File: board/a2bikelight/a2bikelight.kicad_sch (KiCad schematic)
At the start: 1 part

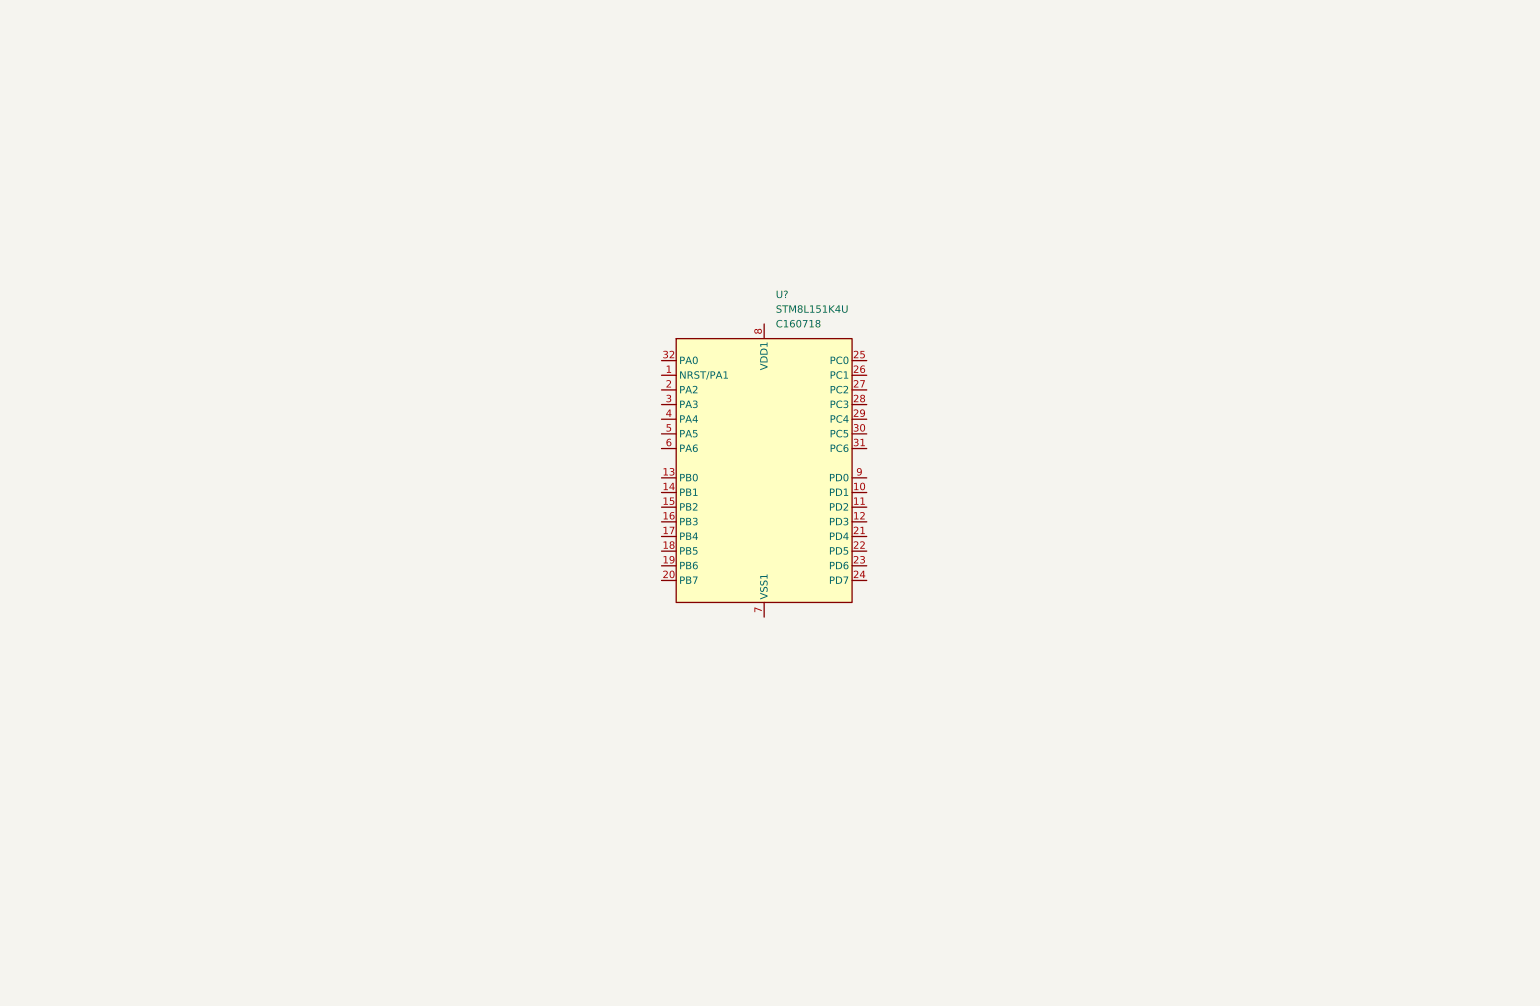
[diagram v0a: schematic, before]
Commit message: baseline
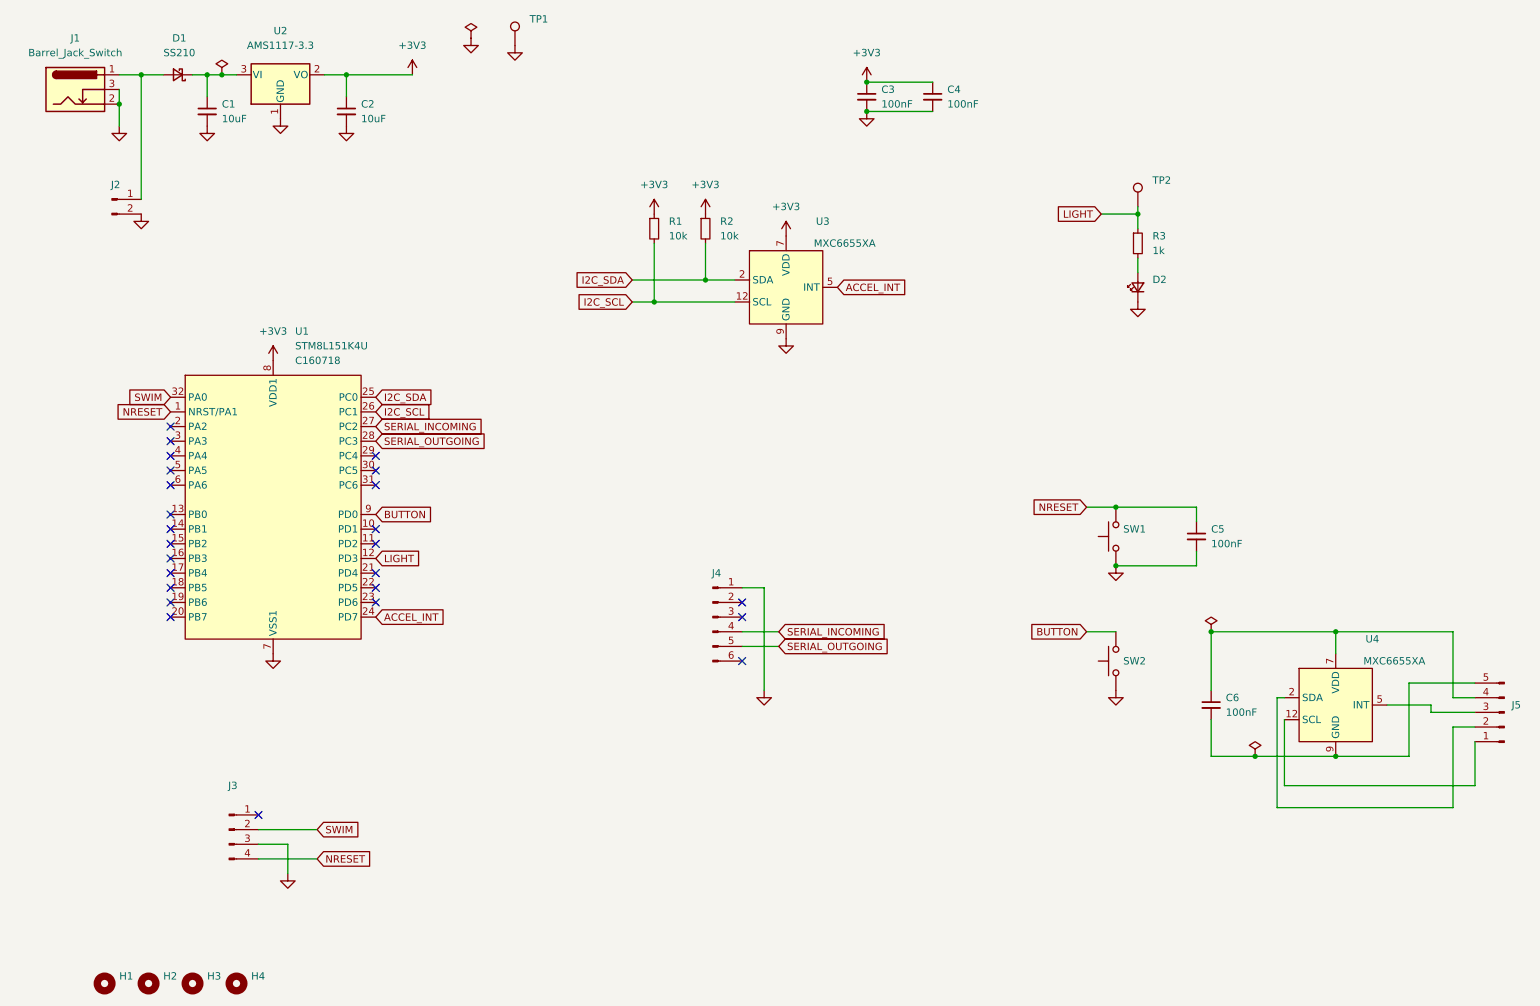
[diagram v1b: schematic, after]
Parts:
- added C1, C2: 10uF, Capacitor_SMD:C_0603_1608Metric, symbol Device:C_Small
- added C3, C4, C5, C6: 100nF, Capacitor_SMD:C_0603_1608Metric, symbol Device:C_Small
- added D1: SS210, Diode_SMD:D_SMA, symbol Device:D_Schottky_Small
- added D2: LED_Small, LED_SMD:LED_0805_2012Metric, symbol Device:LED_Small
- added H1, H2, H3, H4: MountingHole, MountingHole:MountingHole_3.5mm, symbol Mechanical:MountingHole
- added J1: Barrel_Jack_Switch, Connector_BarrelJack:BarrelJack_Horizontal, symbol Connector:Barrel_Jack_Switch
- added J2: Conn_01x02_Male, Connector_PinHeader_2.54mm:PinHeader_1x02_P2.54mm_Vertical, symbol Connector:Conn_01x02_Male
- added J3: Conn_01x04_Male, Connector_PinHeader_2.54mm:PinHeader_1x04_P2.54mm_Vertical, symbol Connector:Conn_01x04_Male
- added J4: Conn_01x06_Male, Connector_PinHeader_2.54mm:PinHeader_1x06_P2.54mm_Vertical, symbol Connector:Conn_01x06_Male
- added J5: Conn_01x05_Male, Connector_PinHeader_2.54mm:PinHeader_1x05_P2.54mm_Vertical, symbol Connector:Conn_01x05_Male
- added R1, R2: 10k, Resistor_SMD:R_0603_1608Metric, symbol Device:R_Small
- added R3: 1k, Resistor_SMD:R_0603_1608Metric, symbol Device:R_Small
- added SW1, SW2: SW_Push, Button_Switch_THT:SW_PUSH_6mm, symbol Switch:SW_Push
- added TP1, TP2: TestPoint, TestPoint:TestPoint_THTPad_2.0x2.0mm_Drill1.0mm, symbol Connector:TestPoint
- added U2: AMS1117-3.3, Package_TO_SOT_SMD:SOT-223-3_TabPin2, symbol Regulator_Linear:AMS1117-3.3
- added U3, U4: MXC6655XA, Package_LGA:LGA-12_2x2mm_P0.5mm, symbol a2bikelight:MXC6655XA
- gave numbers to parts that had none: 1
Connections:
- net NRESET: now reaches U1.1 (NRST/PA1)
- net NRESET: now also C5.1, J3.4 (Pin_4), SW1.2
- net LIGHT: now reaches U1.12 (PD3)
- net LIGHT: now also R3.1, TP2.1
- net ACCEL_INT: now reaches U1.24 (PD7)
- net ACCEL_INT: now also U3.5 (INT)
- net I2C_SDA: now reaches U1.25 (PC0)
- net I2C_SDA: now also R2.2, U3.2 (SDA)
- net I2C_SCL: now reaches U1.26 (PC1)
- net I2C_SCL: now also R1.2, U3.12 (SCL)
- net SERIAL_INCOMING: now reaches U1.27 (PC2)
- net SERIAL_INCOMING: now also J4.4 (Pin_4)
- net SERIAL_OUTGOING: now reaches U1.28 (PC3)
- net SERIAL_OUTGOING: now also J4.5 (Pin_5)
- net SWIM: now reaches U1.32 (PA0)
- net SWIM: now also J3.2 (Pin_2)
- net GND: now reaches U1.7 (VSS1)
- net GND: now also C1.2, C2.2, C3.2, C4.2, C5.2, D2.1 (K), J1.2, J1.3, J2.2 (Pin_2), J3.3 (Pin_3), J4.1 (Pin_1), SW1.1, SW2.1, TP1.1, U2.1 (GND), U3.9 (GND)
- net +3V3: now reaches U1.8 (VDD1)
- net +3V3: now also C2.1, C3.1, C4.1, R1.1, R2.1, U2.2 (VO), U3.7 (VDD)
- net BUTTON: now reaches U1.9 (PD0)
- net BUTTON: now also SW2.2
- new net: D2.2 (A), R3.2
- new net: C1.1, D1.1 (K), U2.3 (VI)
- new net: D1.2 (A), J1.1, J2.1 (Pin_1)
- new net: J5.1 (Pin_1), U4.12 (SCL)
- new net: J5.2 (Pin_2), U4.2 (SDA)
- new net: J5.3 (Pin_3), U4.5 (INT)
- new net: C6.1, J5.4 (Pin_4), U4.7 (VDD)
- new net: C6.2, J5.5 (Pin_5), U4.9 (GND)
- new net thermal: U1.33 (thermal)
- no-connect marks 0 -> 25
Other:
- moved on the sheet: U1
